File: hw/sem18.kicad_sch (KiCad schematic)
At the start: 4 parts, among them J3 USB_C_Receptacle_PowerOnly_6P

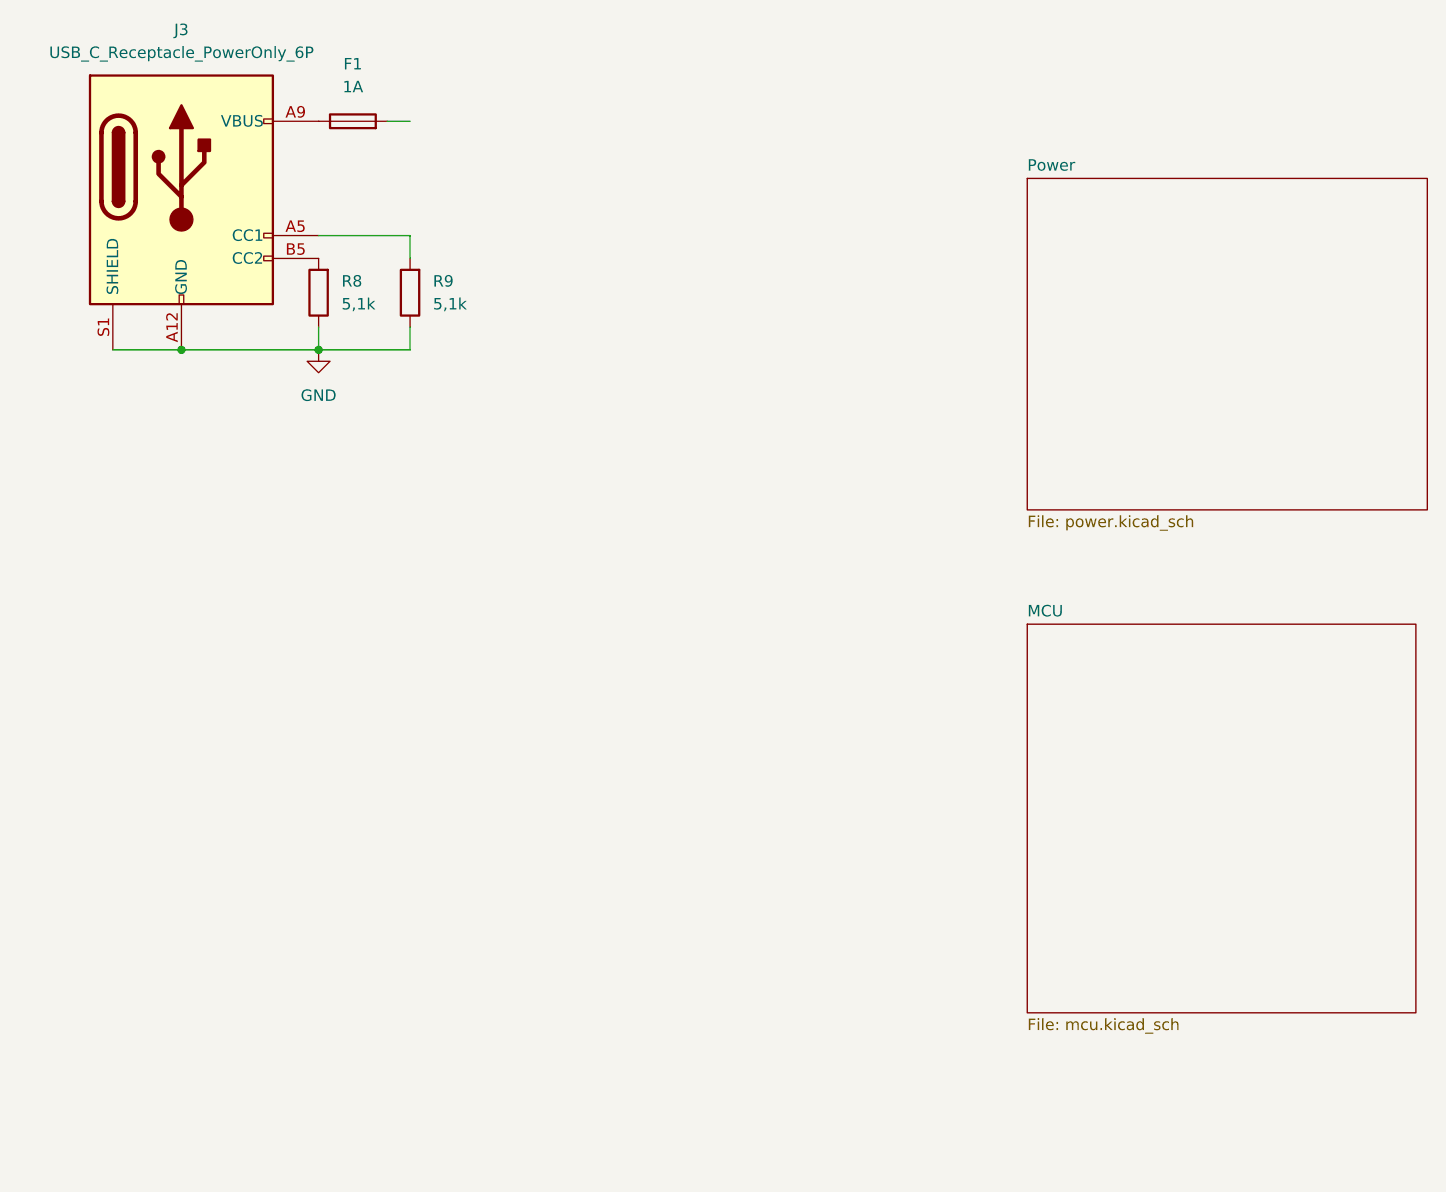
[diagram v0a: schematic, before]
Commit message: WIP
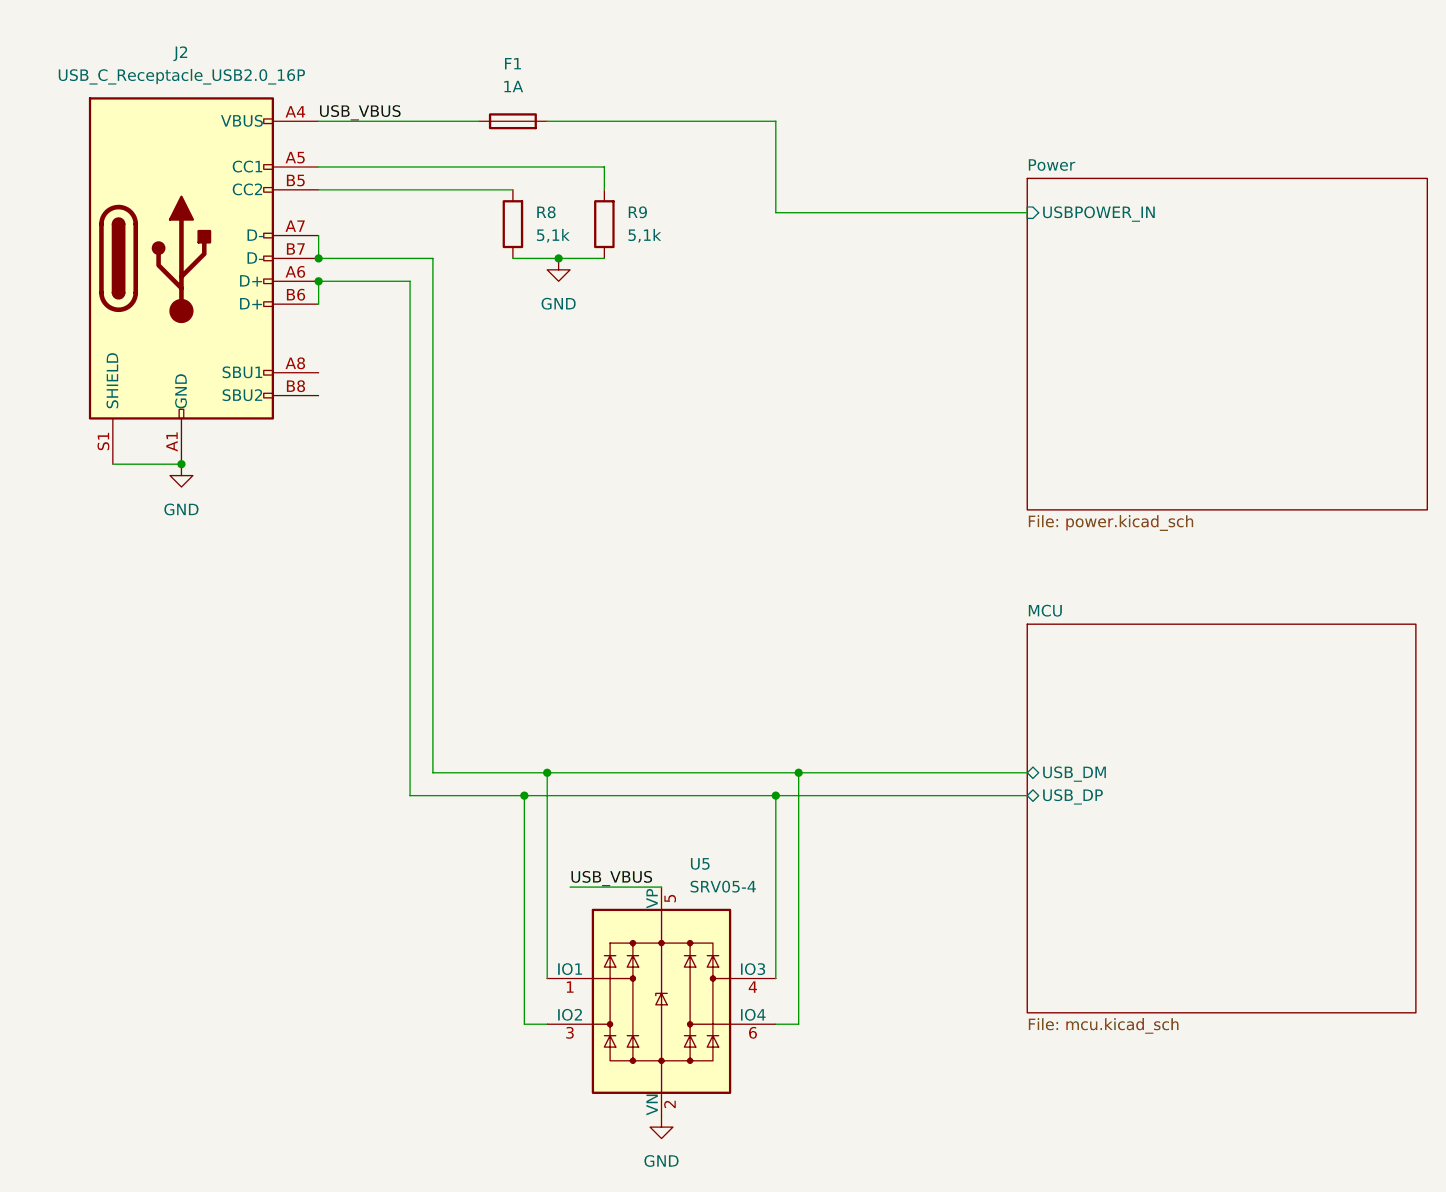
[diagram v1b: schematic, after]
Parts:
- removed J3: USB_C_Receptacle_PowerOnly_6P, Connector_USB:USB_C_Receptacle_GCT_USB4125-xx-x_6P_TopMnt_Horizontal, symbol Connector:USB_C_Receptacle_PowerOnly_6P
- added J2: USB_C_Receptacle_USB2.0_16P, symbol Connector:USB_C_Receptacle_USB2.0_16P
- added U5: SRV05-4, Package_TO_SOT_SMD:SOT-23-6, symbol Power_Protection:SRV05-4
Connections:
- net GND: now also J2.A1 (GND), J2.A12 (GND), J2.B1 (GND), J2.B12 (GND), J2.S1 (SHIELD), U5.2 (VN)
- net at R9.2: now also J2.A5 (CC1)
- net USB_VBUS: now reaches F1.1
- net USB_VBUS: now also J2.A4 (VBUS), J2.A9 (VBUS), J2.B4 (VBUS), J2.B9 (VBUS), U5.5 (VP)
- net at R8.2: now also J2.B5 (CC2)
- net Power/USBPOWER_IN: now reaches F1.2
- new net MCU/USB_DM: J2.A7 (D-), J2.B7 (D-), U5.1 (IO1), U5.6 (IO4)
- new net MCU/USB_DP: J2.A6 (D+), J2.B6 (D+), U5.3 (IO2), U5.4 (IO3)
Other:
- sheet MCU ports: added USB_DM, USB_DP; removed none
- sheet Power ports: added USBPOWER_IN; removed none
- moved on the sheet: F1, R8, R9
